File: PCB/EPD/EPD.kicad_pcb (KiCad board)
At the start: 2 copper layers, 70 x 70 mm, 66 parts, among them J1 Conn_01x26, J2 Shelly, J3 USB-PROG, J4 BTN1, J6 BTN2, J7 USB-C-Socket-V, J8 PWR, P1 +, P10 2, P11 1, P12 1, P2 -, P3 2, P4 2, P5 1, P6 1, P7 +, P8 -, P9 2, Q1 BSS138, U3 MD8942, U4 ESP32-S3-MINI-1

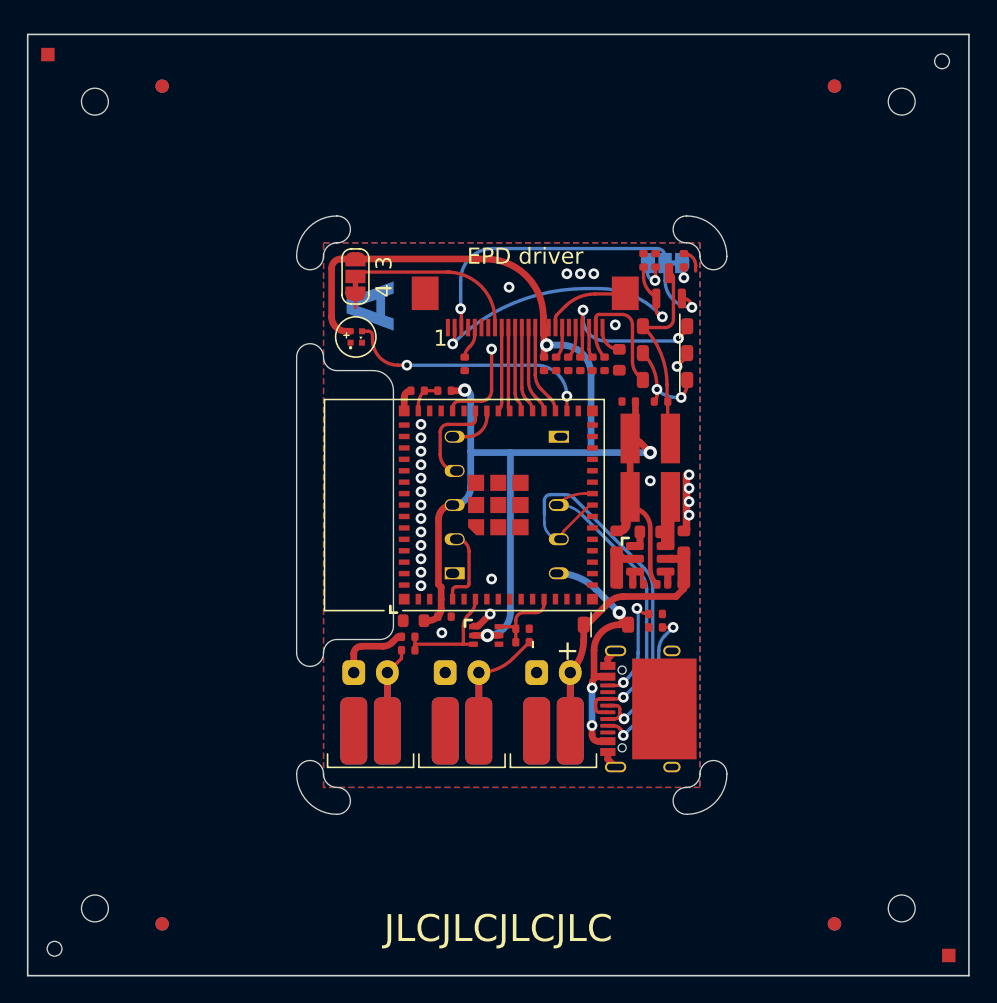
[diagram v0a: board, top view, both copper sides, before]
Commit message: Smaller
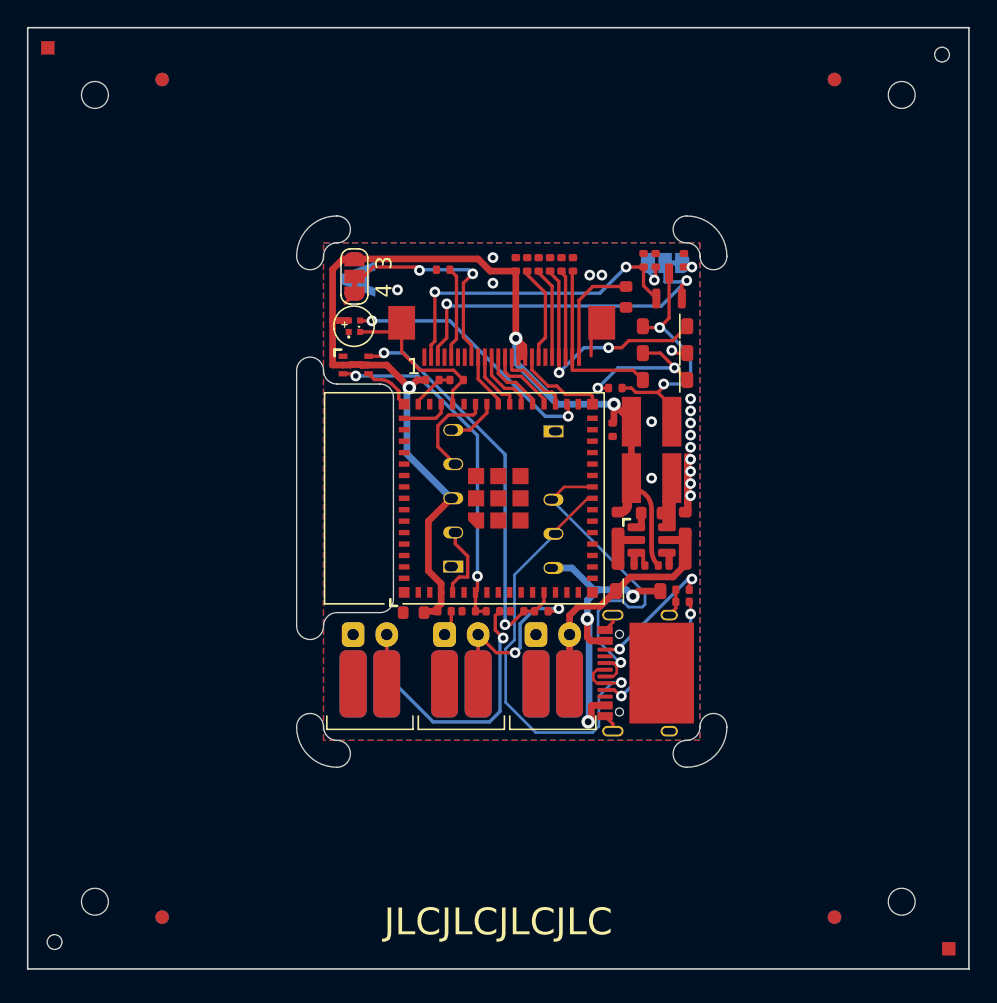
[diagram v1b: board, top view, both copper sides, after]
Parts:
- moved D7 22.3 mm to (88.4, 80.1)
- moved C14 7.76 mm to (104.5, 72.6), turned to 90 degrees
- moved C3 7.75 mm to (103.7, 72.6), turned to 90 degrees
- moved C15 7.73 mm to (102.8, 72.6), turned to 90 degrees
- moved C4 7.72 mm to (102.0, 72.6), turned to 90 degrees
- moved C7 7.71 mm to (101.2, 72.6), turned to 90 degrees
- moved C11 7.69 mm to (100.3, 72.6), turned to 90 degrees
- moved C12 7.18 mm to (94.9, 73.0), turned to 180 degrees
- moved R7 6.94 mm to (98.6, 98.4), turned to 180 degrees
- moved C22 4.88 mm to (96.8, 98.4)
- moved C1 4.70 mm to (108.5, 75.0)
- moved C17 3.54 mm to (107.7, 81.8)
- moved P1 3.50 mm to (104.3, 103.8)
- moved P10 3.50 mm to (95.0, 103.8)
- moved P11 3.50 mm to (90.7, 103.8)
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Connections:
- U4 pad 9: unconnected-(U4-GPIO5-Pad9) -> GND
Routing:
- net BTN2: track 6.06 -> 30.3 mm, vias 0 -> 2
- net +3.3V: track 96.0 -> 77.5 mm, vias 4 -> 3
- net BTN1: track 8.86 -> 25.8 mm, vias 0 -> 2
- net Net-(J4-Pin_2): track 10.8 -> 24.8 mm, vias 0 -> 1
- net GND: track 28.3 -> 37.8 mm, vias 28 -> 17
- net Net-(J1-Pin_24): track 1.91 -> 8.15 mm
- net Net-(D3-K): track 12.9 -> 18.6 mm
- net Net-(D1-A): track 7.06 -> 12.6 mm
- net Net-(J1-Pin_18): track 2.24 -> 7.17 mm
- net VBUS: track 20.0 -> 24.5 mm
- net Net-(J1-Pin_20): track 2.34 -> 6.69 mm
- net Net-(J1-Pin_5): track 2.41 -> 6.72 mm
- net Net-(J1-Pin_22): track 2.26 -> 6.40 mm
- net Net-(J6-Pin_2): track 13.2 -> 17.2 mm, vias 0 -> 2
- net PWR: track 22.5 -> 18.9 mm
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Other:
- board text removed: "+"
- board text removed: "-"
- board text removed: "EPD driver"
